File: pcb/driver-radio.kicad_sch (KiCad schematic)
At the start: 37 parts, among them J3 Conn_01x02_MountingPin, J4 Conn_01x02_MountingPin, J6 Conn_Coaxial

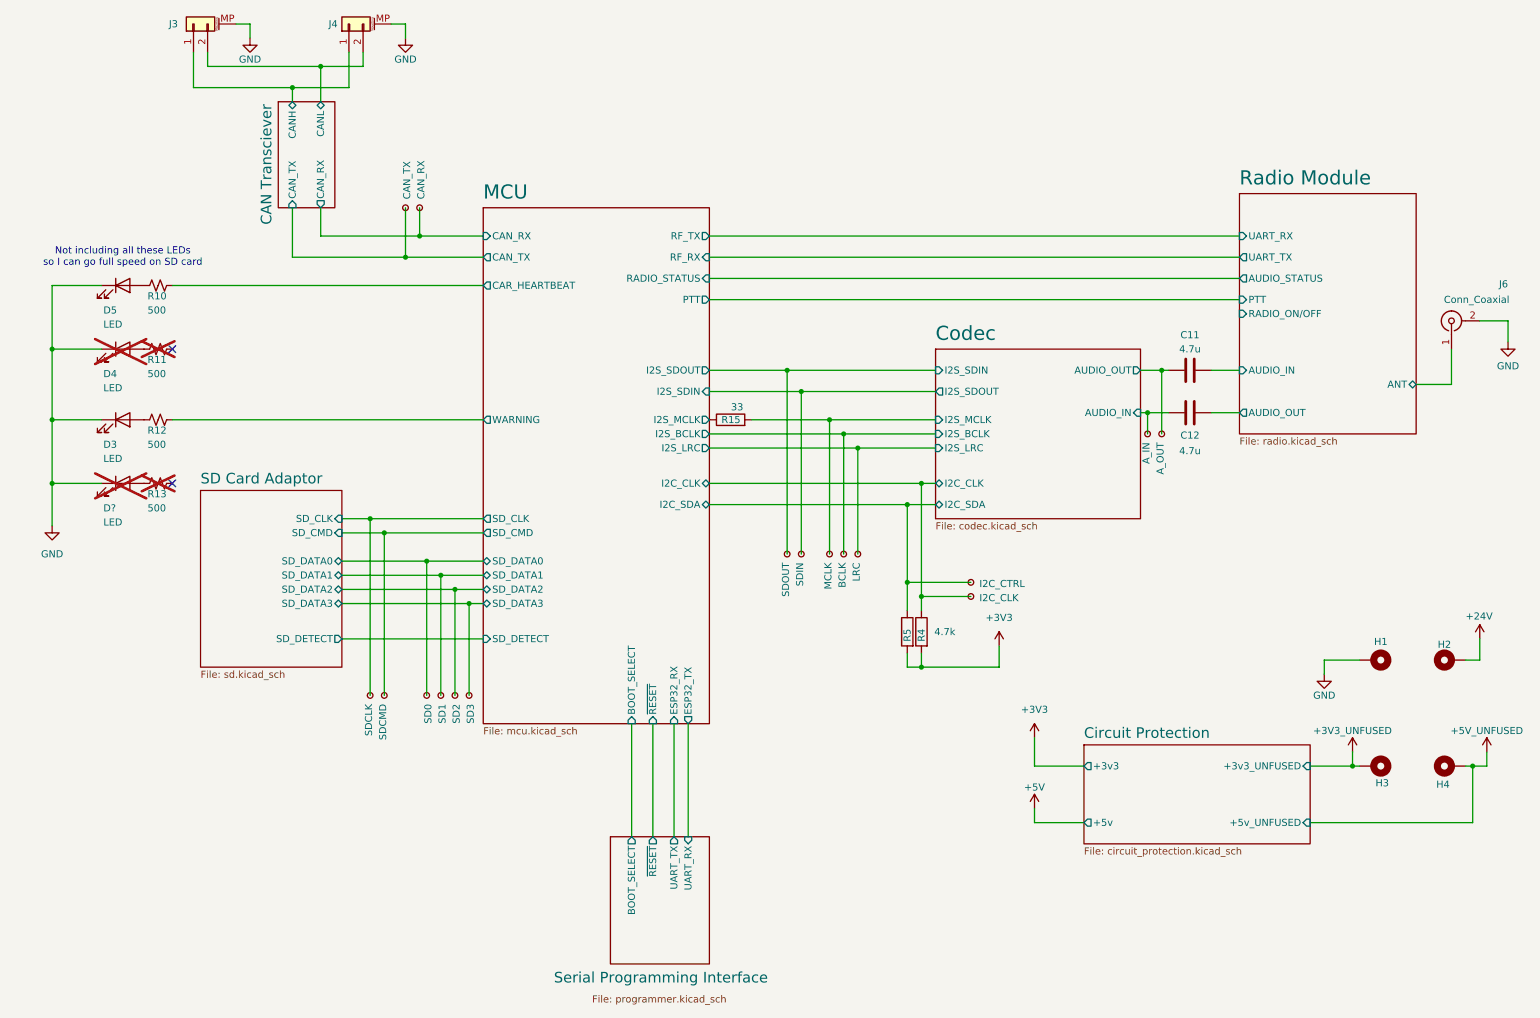
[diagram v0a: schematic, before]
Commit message: Merging in work from FSAE repo from when I forgot this one existed
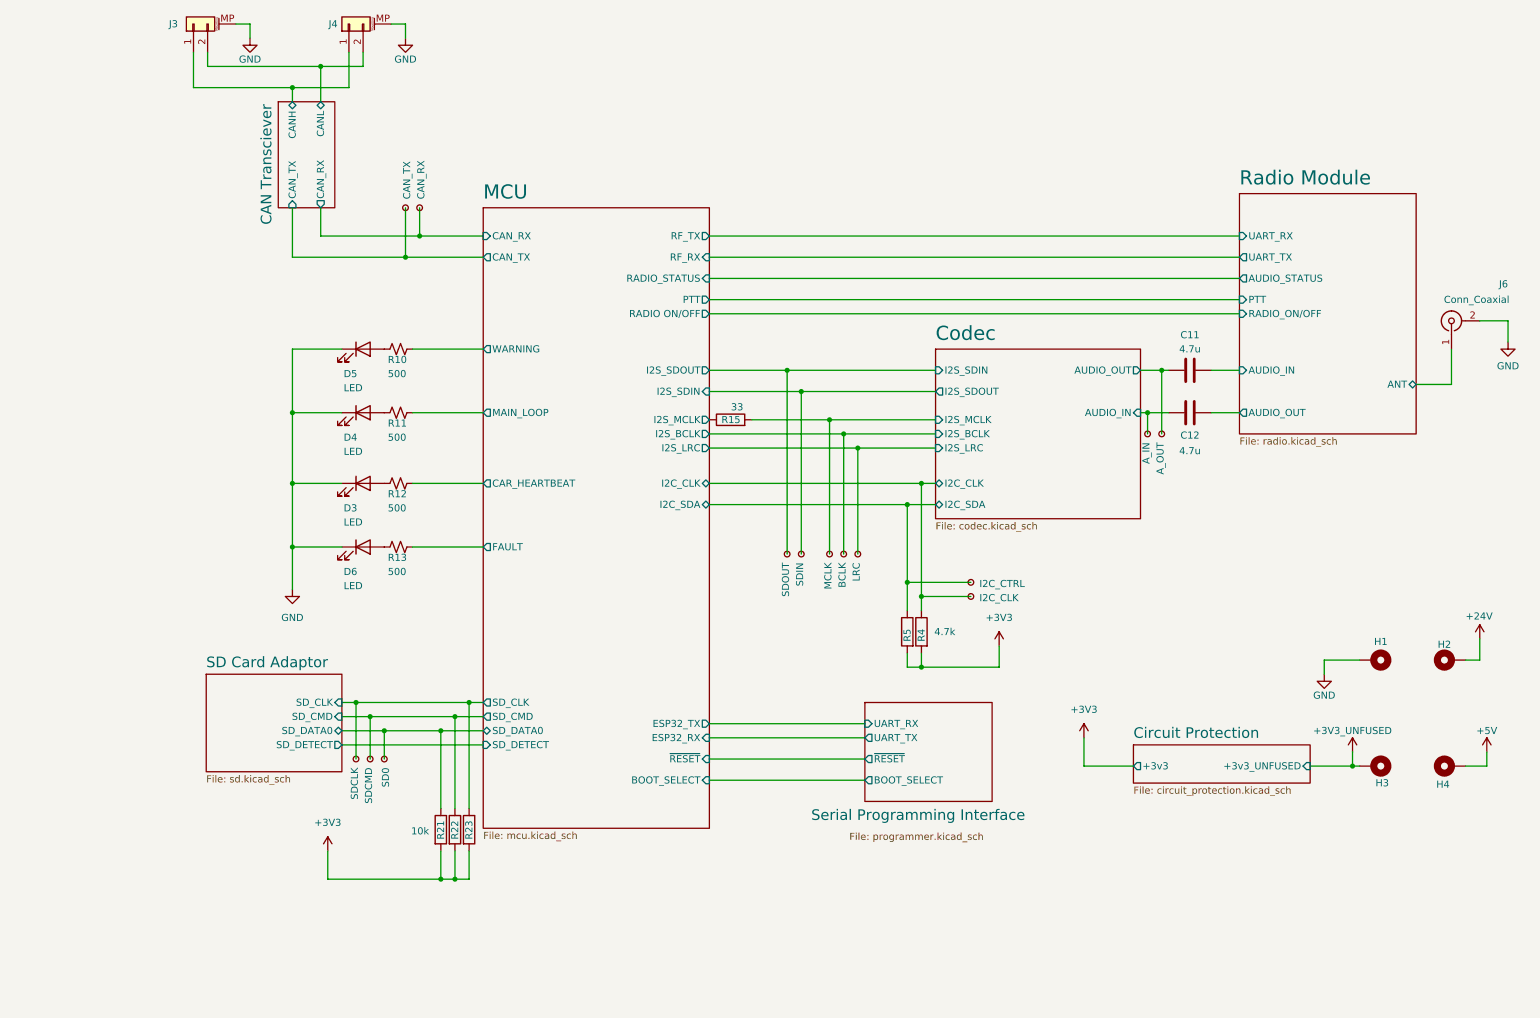
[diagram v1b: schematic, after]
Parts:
- removed TP13: SD1, ev24-footprint-library:tp-ev24-nobacksilk, symbol Connector:TestPoint_Small
- removed TP14: SD2, ev24-footprint-library:tp-ev24-nobacksilk, symbol Connector:TestPoint_Small
- removed TP15: SD3, ev24-footprint-library:tp-ev24-nobacksilk, symbol Connector:TestPoint_Small
- added R21, R22, R23: 10k, Resistor_SMD:R_0402_1005Metric_Pad0.72x0.64mm_HandSolder, symbol Device:R
- D3, D5: footprint (none) -> LED_SMD:LED_0402_1005Metric
- D4: footprint (none) -> LED_SMD:LED_0402_1005Metric; now fitted; now in the parts list
- D6: renamed from D?; footprint (none) -> LED_SMD:LED_0402_1005Metric; now fitted; now in the parts list
- R11, R13: now fitted; now in the parts list
- TP1, TP10, TP12, TP16, TP2, TP3, TP4, TP5, TP6, TP7, TP8, TP9: footprint ev24-footprint-library:tp-ev24-nobacksilk -> 0_tp-ev24-nobacksilk:tp-ev24-nobacksilk
- TP11, TP17: footprint TestPoint:TestPoint_Pad_1.0x1.0mm -> 0_tp-ev24-nobacksilk:tp-ev24-nobacksilk
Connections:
- net +5V_UNFUSED is gone; now on net +5V: H4.1
- net +3V3: now also R21.2, R22.2, R23.2
- net MCU/CAR_HEARTBEAT: now also R12.1; no longer R10.1
- net MCU/SD_CLK: now also R23.1
- net MCU/SD_CMD: now also R22.1
- net MCU/SD_DATA0: now also R21.1
- net MCU/WARNING: now also R10.1; no longer R12.1
- net MCU/MAIN_LOOP: now reaches R11.1
- net MCU/FAULT: now reaches R13.1
- no-connect marks 2 -> 0
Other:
- sheet Circuit Protection ports: added none; removed +5v, +5v_UNFUSED
- sheet MCU ports: added FAULT, MAIN_LOOP, RADIO ON/OFF; removed SD_DATA1, SD_DATA2, SD_DATA3
- sheet SD Card Adaptor ports: added none; removed SD_DATA1, SD_DATA2, SD_DATA3
- note removed: "Not including all these LEDs so I can go full speed on SD card"
- moved on the sheet: D3, D5, R10, R12
